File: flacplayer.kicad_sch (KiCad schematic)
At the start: 68 parts, among them J1 AudioJack3, J2 USB_C_Receptacle_USB2.0, J3 Micro_SD_Card, J4 Conn_01x24_MountingPin, Q1 DMG3414U, Q2 AO3400A, SW1 SW_Push, SW2 SW_Push, SW3 SW_Push, SW4 SW_Push, SW5 SW_Push, SW6 SW_Push, SW7 SW_Push, U1 ESP32-S3-MINI-1, U2 MAX17048X, U3 AMS1117-3.3, U5 TAD5242, U6 TPA6132A2RTE, U7 MCP73831-2-OT

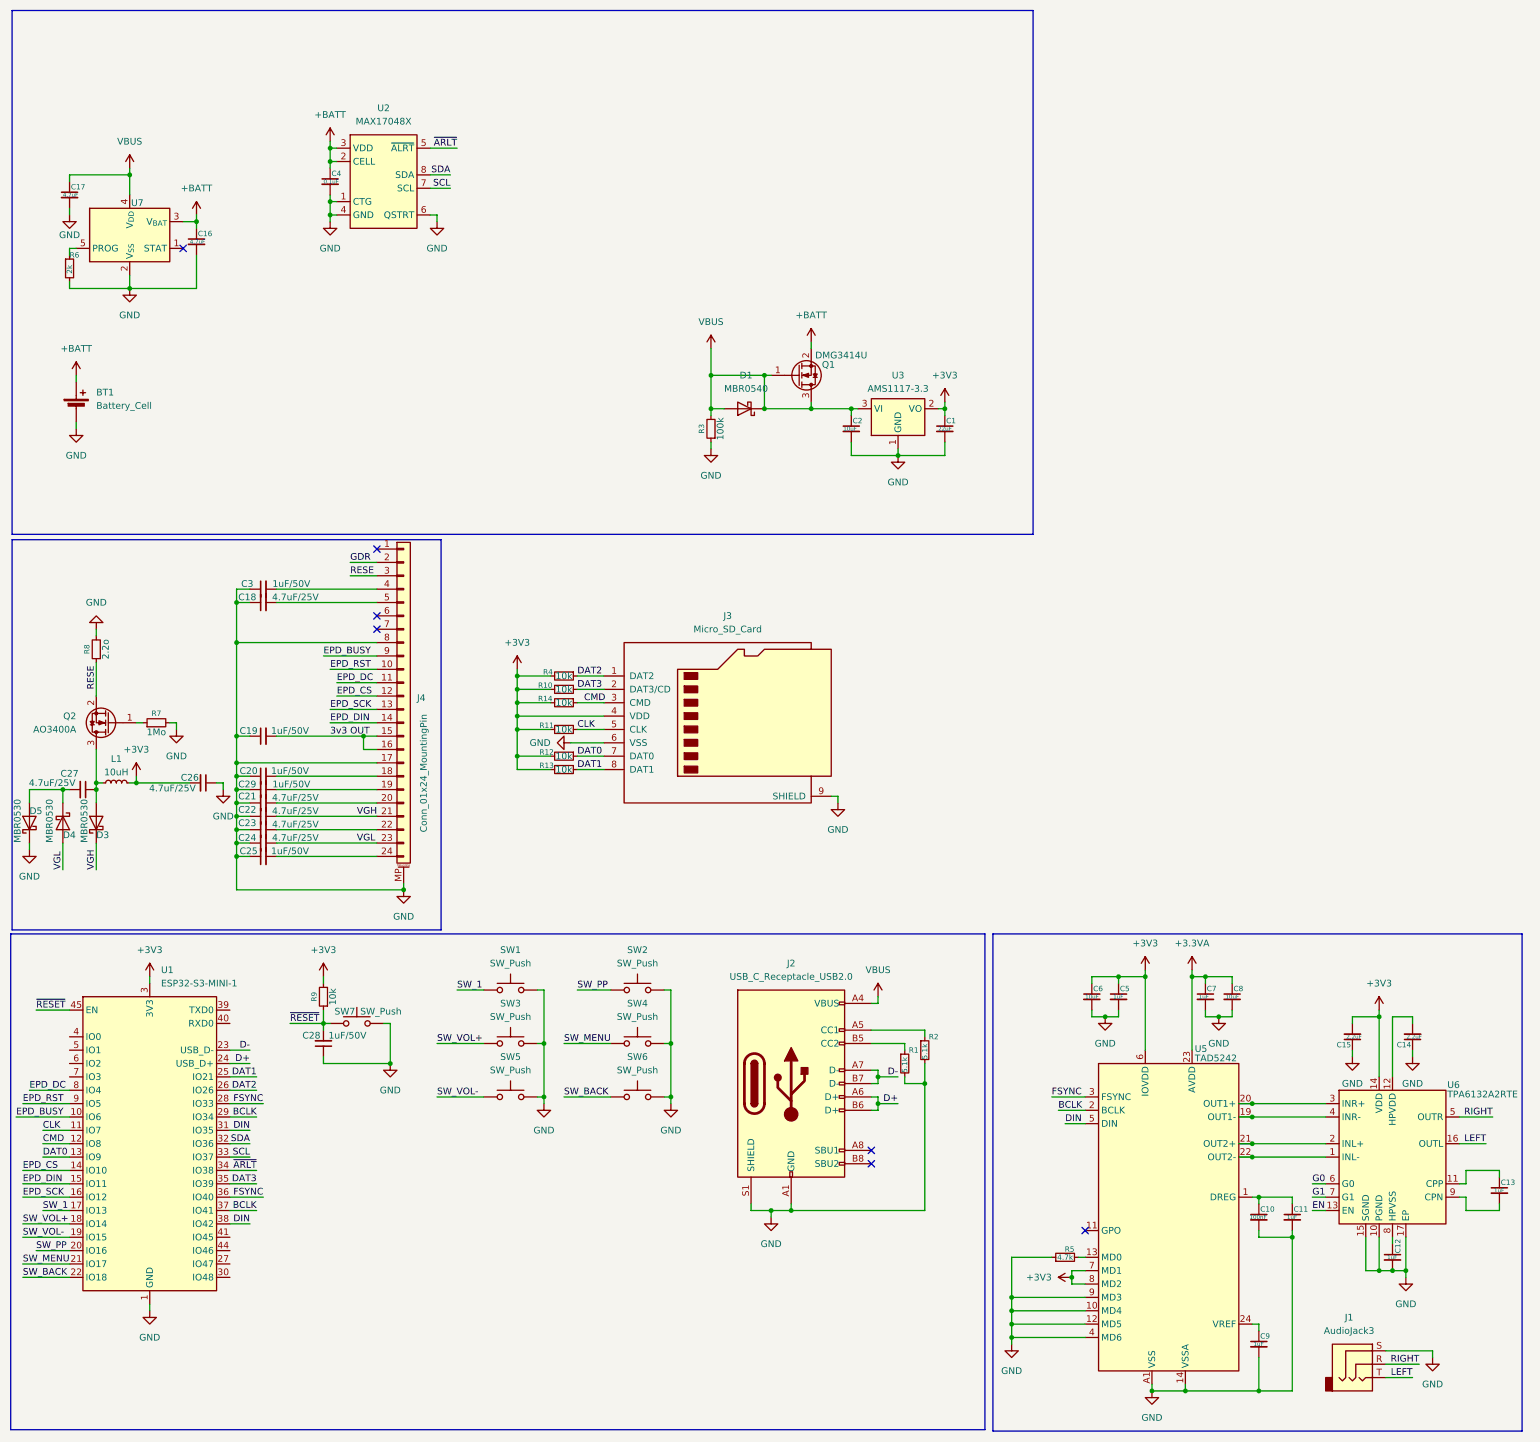
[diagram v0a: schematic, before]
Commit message: fix component issues
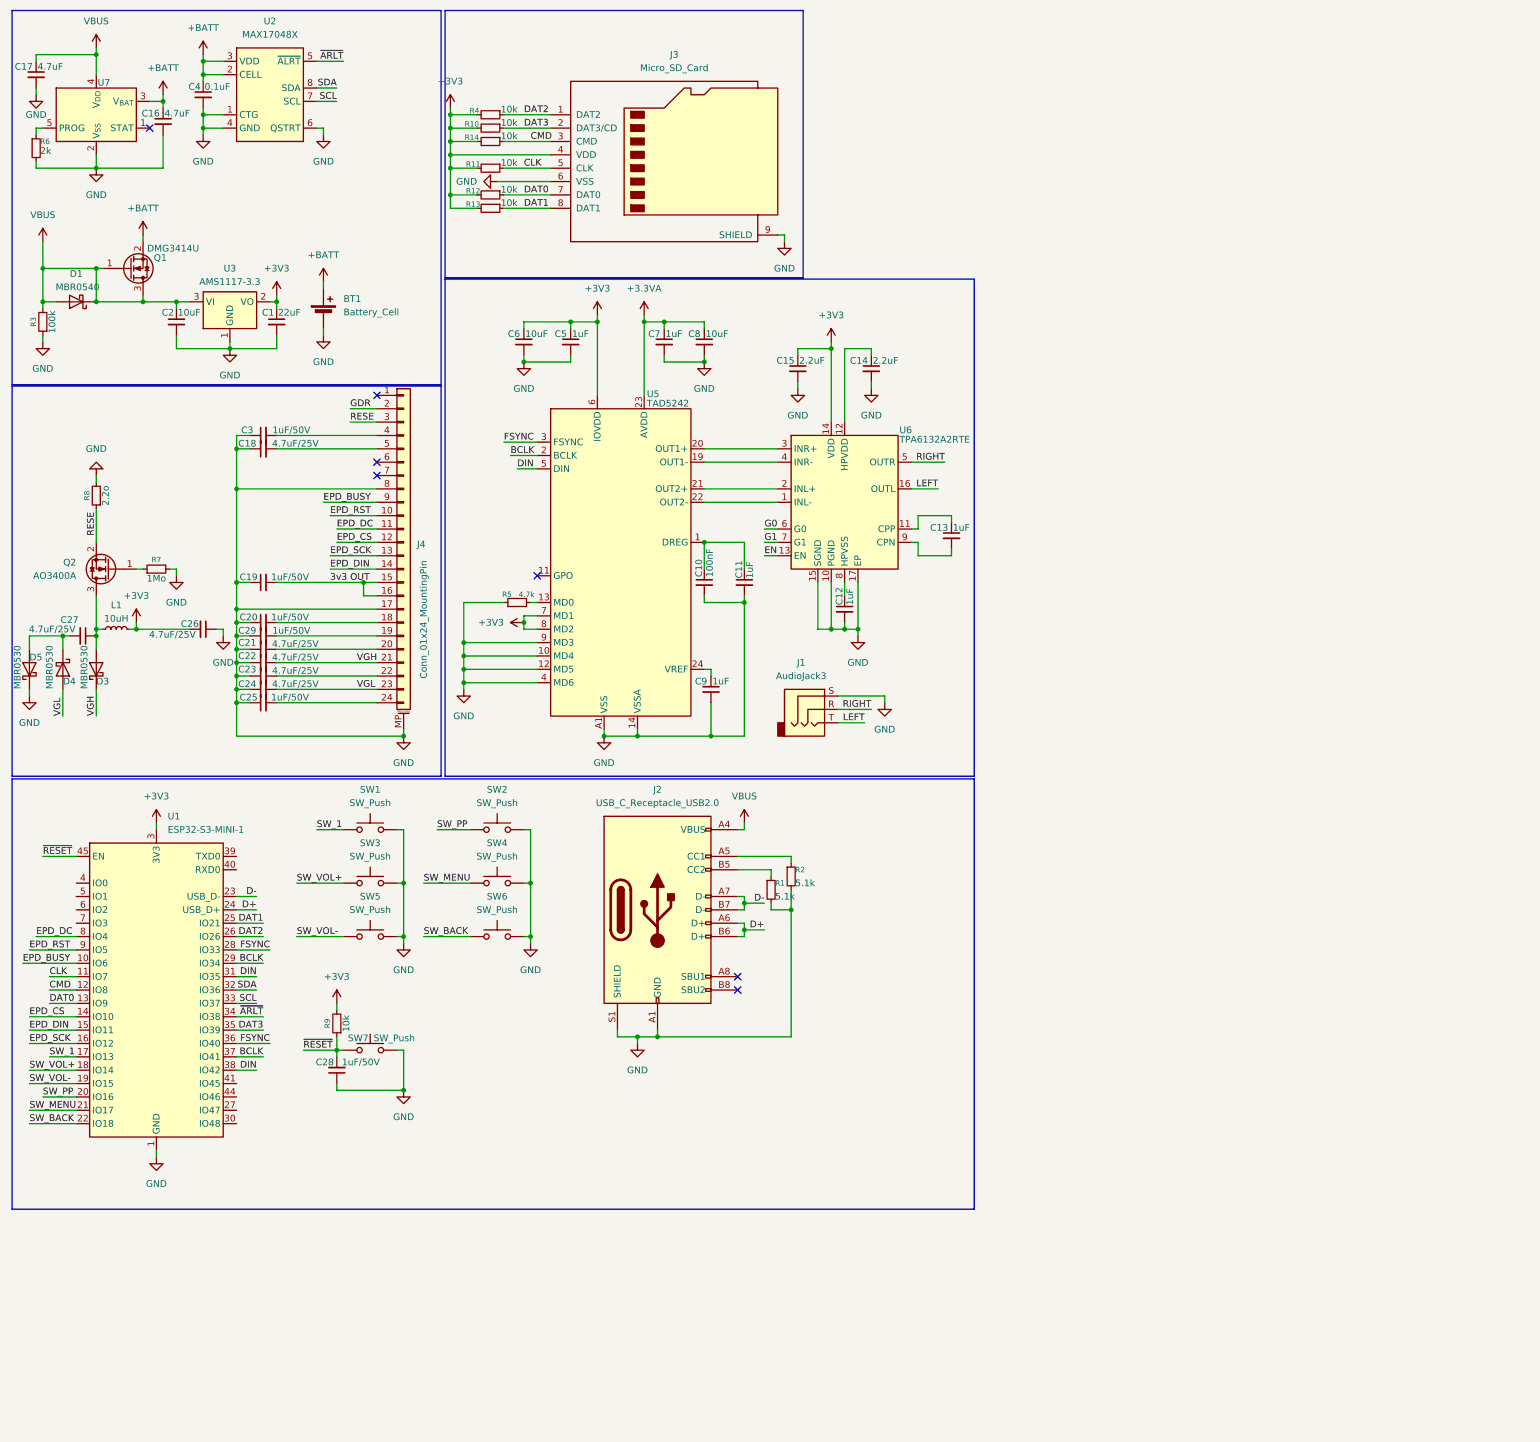
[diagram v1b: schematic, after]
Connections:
- net +3V3: now also C15.1; no longer C15.2
- net GND: now also C14.2, C15.2; no longer C14.1, C15.1
- net at U6.12 (HPVDD): now also C14.1; no longer C14.2
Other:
- moved on the sheet: BT1, C18, C19, C20, C21, C22, C23, C24, C25, C26, C27, C28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
